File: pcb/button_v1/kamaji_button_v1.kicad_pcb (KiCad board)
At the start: 2 copper layers, 30 x 35 mm, 4 parts, among them J1 RJ10, SW2 SW_Push_LED

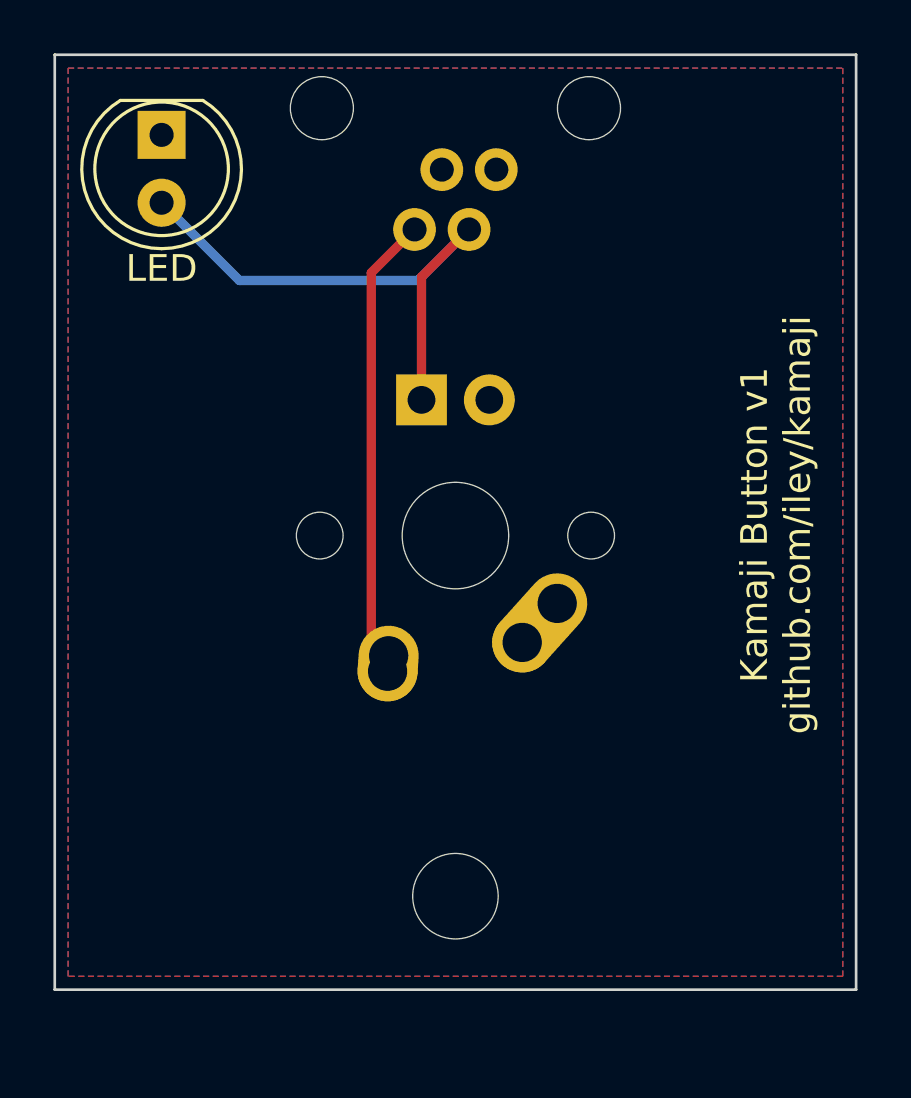
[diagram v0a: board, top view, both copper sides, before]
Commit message: Fix CI
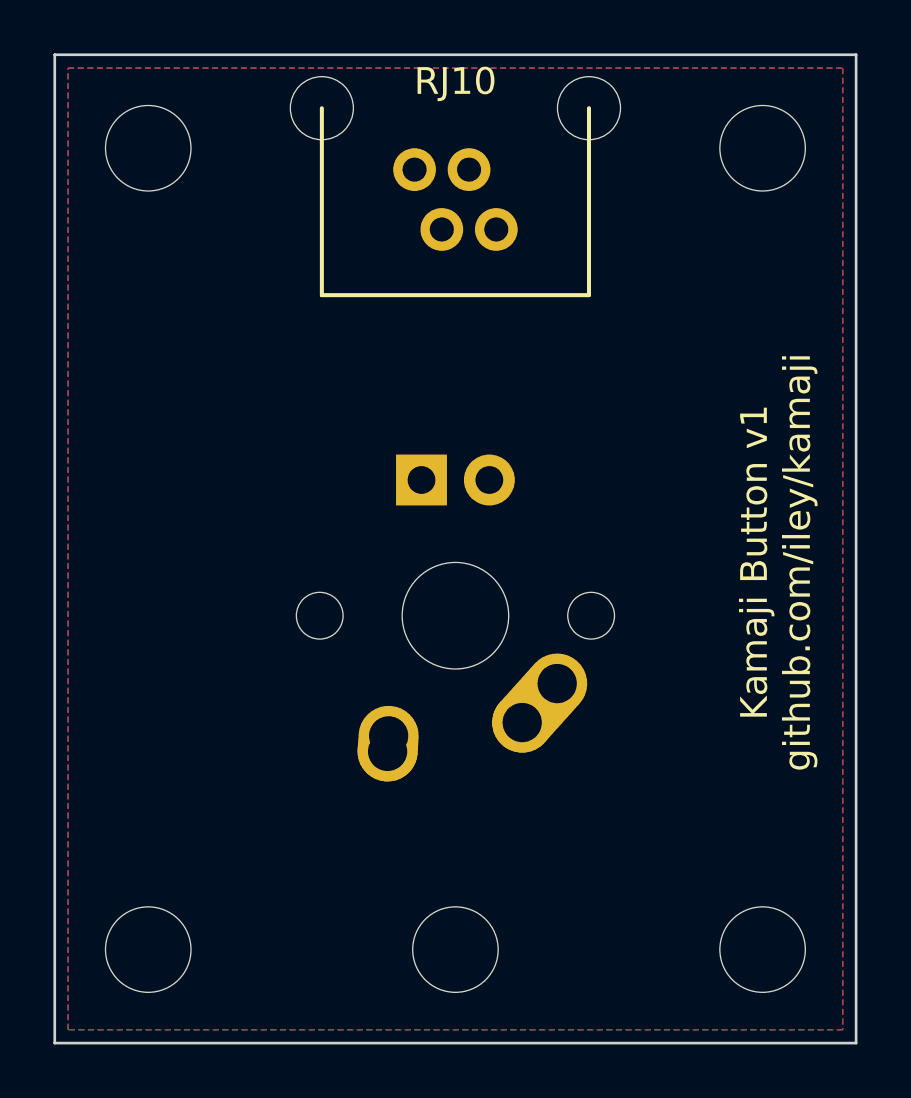
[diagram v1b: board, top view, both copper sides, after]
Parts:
- removed D1: LED, LED_THT:LED_D5.0mm
- added REF**: MountingHole_3.2mm_M3, MountingHole:MountingHole_3.2mm_M3, F.Cu at (76.5, 83.5)
- added REF**: MountingHole_3.2mm_M3, MountingHole:MountingHole_3.2mm_M3, F.Cu at (53.5, 83.5)
- added REF**: MountingHole_3.2mm_M3, MountingHole:MountingHole_3.2mm_M3, F.Cu at (53.5, 53.5)
- added REF**: MountingHole_3.2mm_M3, MountingHole:MountingHole_3.2mm_M3, F.Cu at (76.5, 53.5)
- J1: moved to F.Cu
- moved SW2 3.00 mm to (65.0, 71.0)
- moved REF** 2.00 mm to (65.0, 83.5)
- turned J1 to 180 degrees
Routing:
- net Net-(J1-Pad2): track 20.6 -> 0.00 mm
- net Net-(J1-Pad4): track 16.9 -> 0.00 mm
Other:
- board size 30 x 35 mm -> 30 x 37 mm
